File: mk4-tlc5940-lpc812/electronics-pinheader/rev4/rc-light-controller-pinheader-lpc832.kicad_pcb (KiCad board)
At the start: 2 copper layers, 44 x 23 mm, 14 parts, among them J1 Pinheader right-angle 2x17, J2 Pinheader straight 1x06, J3 Pinheader straight 1x06, T9 PMV30UN, U1 LPC832M101FDH20, U2 TLC5940PWP, U3 MCP1703A-3302_SOT23

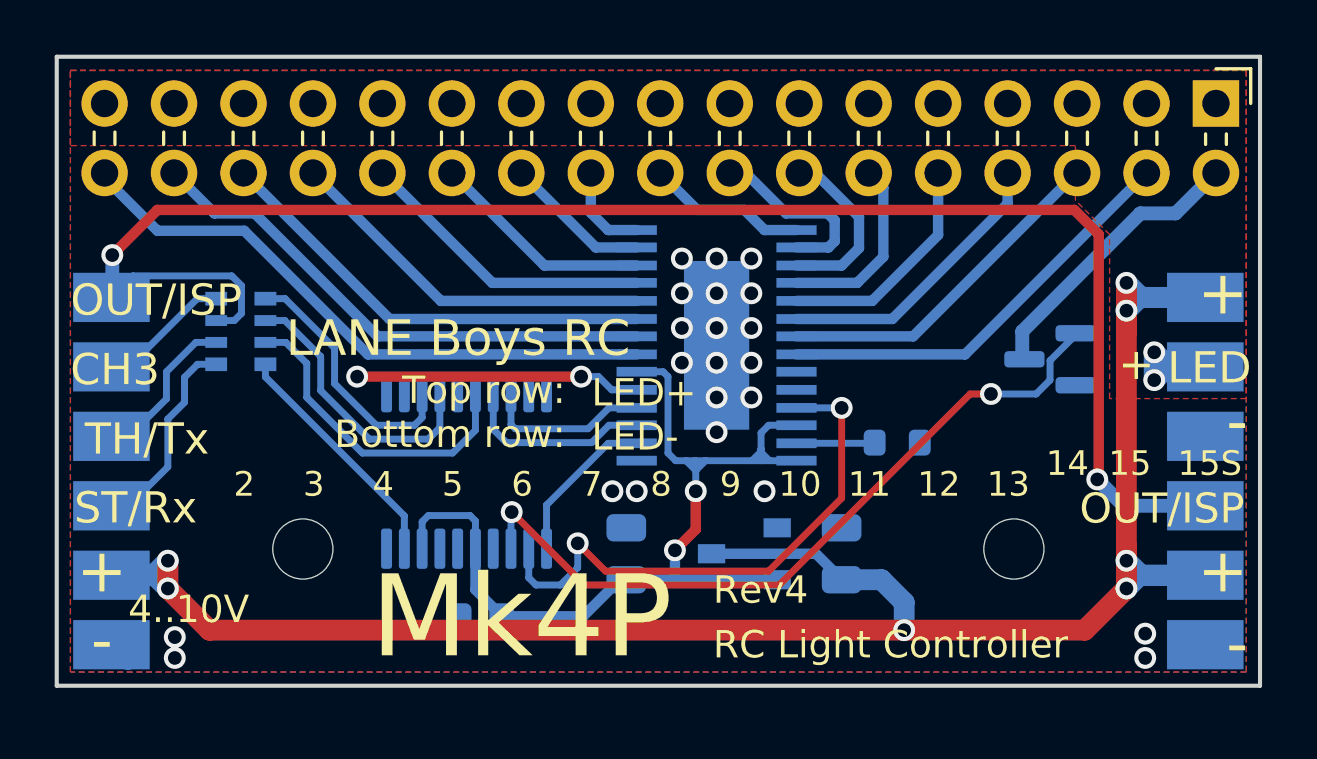
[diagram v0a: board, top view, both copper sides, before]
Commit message: Fix layout and pass DRC
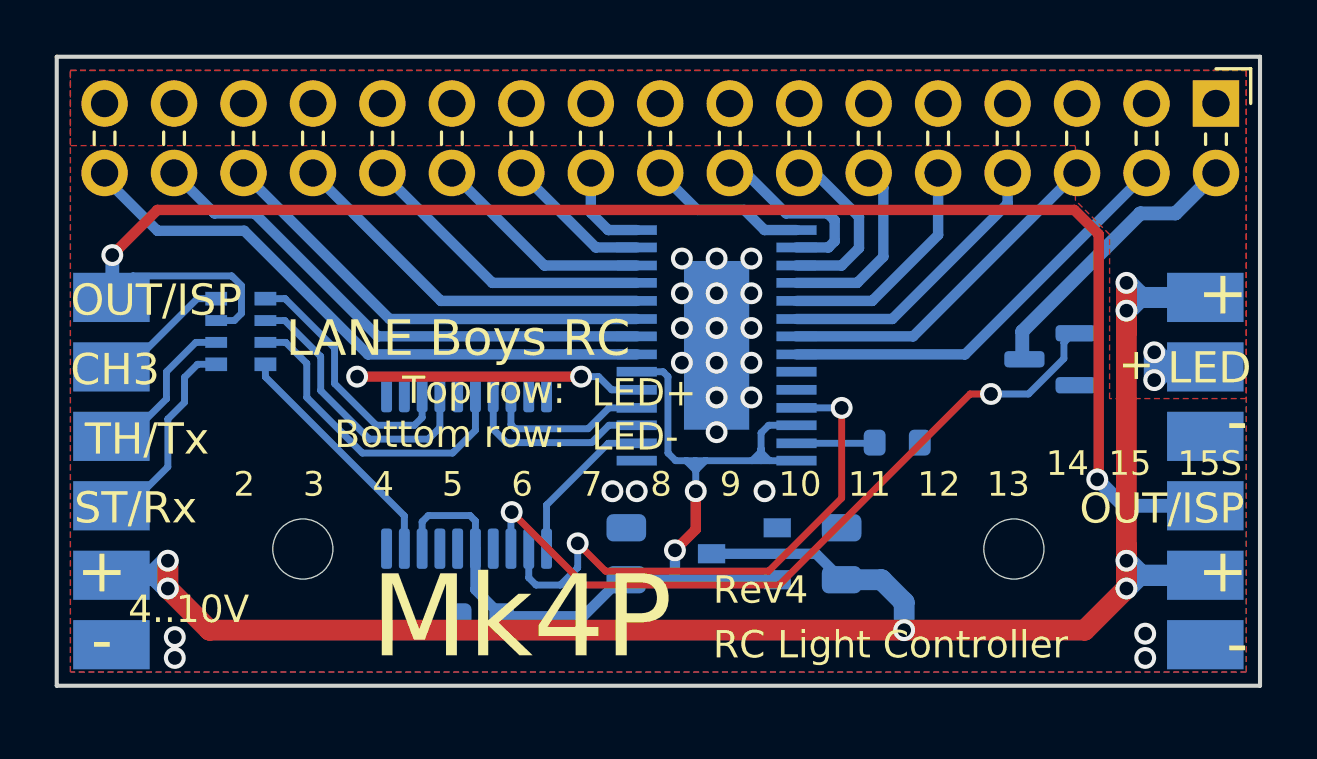
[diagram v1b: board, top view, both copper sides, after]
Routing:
- net /OUT-ISP-out: track 61.9 -> 59.3 mm
- net GND: track 1.85 -> 0.21 mm
- net /CH3-in: track 4.94 -> 4.22 mm
- net /ST-Rx-in: track 7.57 -> 6.89 mm
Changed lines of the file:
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@@
     (fp_line (start 1.042929 28.32) (end 1.497071 28.32) (layer "F.SilkS") (width 0.12))
     (fp_line (start 1.042929 8) (end 1.497071 8) (layer "F.SilkS") (width 0.12))
-    (fp_line (start -1.8 -1.8) (end -1.8 42.45) (layer "F.CrtYd") (width 0.05))
     (fp_line (start -0.32 40.32) (end -0.32 40.96) (layer "F.Fab") (width 0.1))
     (fp_line (start -0.32 2.22) (end -0.32 2.86) (layer "F.Fab") (width 0.1))
@@
   (via (at 157.606 109.047) (size 0.8) (drill 0.5) (layers "F.Cu" "B.Cu") (net 1))
   (segment (start 157.6314 105.7704) (end 157.352 105.491) (width 0.254) (layer "B.Cu") (net 1))
+  (segment (start 150.113 107.777) (end 150.311 107.975) (width 0.254) (layer "B.Cu") (net 1))
+  (segment (start 148.361 108.9885) (end 148.361 108.005) (width 0.254) (layer "B.Cu") (net 1))
   (segment (start 158.368 106.126) (end 158.0124 105.7704) (width 0.254) (layer "B.Cu") (net 1))
   (segment (start 160.4254 105.7704) (end 158.7236 105.7704) (width 0.254) (layer "B.Cu") (net 1))
   (segment (start 161.3398 110.1138) (end 155.8303 110.1138) (width 0.381) (layer "B.Cu") (net 1))
+  (segment (start 148.589 107.777) (end 150.113 107.777) (width 0.254) (layer "B.Cu") (net 1))
   (segment (start 161.035 104.475) (end 160.7556 104.7544) (width 0.254) (layer "B.Cu") (net 1))
   (segment (start 154.2532 111.46) (end 155.6017 110.1115) (width 0.381) (layer "B.Cu") (net 1))
   (segment (start 160.7556 105.4402) (end 160.4254 105.7704) (width 0.254) (layer "B.Cu") (net 1))
   (segment (start 160.7556 105.3386) (end 160.7556 105.4402) (width 0.254) (layer "B.Cu") (net 1))
-  (segment (start 150.113 107.777) (end 150.311 107.975) (width 0.254) (layer "B.Cu") (net 1))
-  (segment (start 148.361 108.9885) (end 148.361 108.692) (width 0.254) (layer "B.Cu") (net 1))
   (segment (start 160.7556 105.4656) (end 161.0604 105.7704) (width 0.254) (layer "B.Cu") (net 1))
   (segment (start 158.368 106.126) (end 158.368 105.7958) (width 0.254) (layer "B.Cu") (net 1))
   (segment (start 158.7236 105.7704) (end 158.3426 105.7704) (width 0.254) (layer "B.Cu") (net 1))
-  (segment (start 148.589 107.777) (end 150.113 107.777) (width 0.254) (layer "B.Cu") (net 1))
   (segment (start 157.352 105.491) (end 157.352 102.697) (width 0.254) (layer "B.Cu") (net 1))
-  (segment (start 158.368 106.888) (end 158.368 106.761) (width 0.254) (layer "B.Cu") (net 1))
+  (segment (start 148.361 108.005) (end 148.589 107.777) (width 0.254) (layer "B.Cu") (net 1))
   (segment (start 157.352 102.697) (end 157.1742 102.5192) (width 0.254) (layer "B.Cu") (net 1))
+  (segment (start 158.368 106.888) (end 158.368 106.126) (width 0.254) (layer "B.Cu") (net 1))
   (segment (start 158.0124 105.7704) (end 157.6314 105.7704) (width 0.254) (layer "B.Cu") (net 1))
-  (segment (start 158.368 106.888) (end 158.368 106.126) (width 0.254) (layer "B.Cu") (net 1))
   (segment (start 162.051 105.7704) (end 161.0604 105.7704) (width 0.254) (layer "B.Cu") (net 1))
   (segment (start 155.6017 110.1115) (end 155.828 110.1115) (width 0.381) (layer "B.Cu") (net 1))
@@
   (segment (start 150.311 110.4895) (end 151.2815 111.46) (width 0.381) (layer "B.Cu") (net 1))
   (segment (start 160.7556 105.7704) (end 160.4254 105.7704) (width 0.254) (layer "B.Cu") (net 1))
+  (segment (start 150.311 107.975) (end 150.311 108.9885) (width 0.254) (layer "B.Cu") (net 1))
   (segment (start 157.1742 102.5192) (end 156.209 102.5192) (width 0.254) (layer "B.Cu") (net 1))
-  (segment (start 148.361 108.005) (end 148.589 107.777) (width 0.254) (layer "B.Cu") (net 1))
   (segment (start 151.2815 111.46) (end 154.2532 111.46) (width 0.381) (layer "B.Cu") (net 1))
   (segment (start 158.3426 105.7704) (end 158.0124 105.7704) (width 0.254) (layer "B.Cu") (net 1))
   (segment (start 158.368 106.126) (end 158.7236 105.7704) (width 0.254) (layer "B.Cu") (net 1))
-  (segment (start 148.361 108.9885) (end 148.361 108.005) (width 0.254) (layer "B.Cu") (net 1))
   (segment (start 160.7556 105.3386) (end 160.7556 105.7704) (width 0.254) (layer "B.Cu") (net 1))
-  (segment (start 150.311 107.975) (end 150.311 108.9885) (width 0.254) (layer "B.Cu") (net 1))
   (segment (start 160.7556 104.7544) (end 160.7556 105.3386) (width 0.254) (layer "B.Cu") (net 1))
   (segment (start 158.368 105.7958) (end 158.3426 105.7704) (width 0.254) (layer "B.Cu") (net 1))
@@
   (via (at 160.4 103.459) (size 0.8) (drill 0.5) (layers "F.Cu" "B.Cu") (net 2))
   (segment (start 137.151 112.349) (end 137 112.5) (width 0.762) (layer "B.Cu") (net 2))
-  (segment (start 137.611 113.111) (end 137 112.5) (width 0.635) (layer "B.Cu") (net 2))
-  (segment (start 137.77 112.5) (end 137 112.5) (width 0.635) (layer "B.Cu") (net 2))
   (segment (start 174.116 110.444) (end 174.116 108.92) (width 0.762) (layer "F.Cu") (net 3))
   (segment (start 140.588 111.968) (end 139.064 110.444) (width 0.762) (layer "F.Cu") (net 3))
@@
   (segment (start 139.064 105.999) (end 139.064 104.2464) (width 0.254) (layer "B.Cu") (net 18))
   (segment (start 140.15 102.246) (end 140.831 102.246) (width 0.254) (layer "B.Cu") (net 18))
-  (segment (start 137 107.42) (end 137.643 107.42) (width 0.254) (layer "B.Cu") (net 18))
-  (segment (start 137.024 107.396) (end 137 107.42) (width 0.762) (layer "B.Cu") (net 18))
   (segment (start 139.6736 103.6368) (end 139.6736 102.7224) (width 0.254) (layer "B.Cu") (net 18))
   (segment (start 137.643 107.42) (end 139.064 105.999) (width 0.254) (layer "B.Cu") (net 18))
@@
   (segment (start 140.0864 101.446) (end 140.831 101.446) (width 0.254) (layer "B.Cu") (net 19))
   (segment (start 137 104.88) (end 137.643 104.88) (width 0.254) (layer "B.Cu") (net 19))
-  (segment (start 137 102.34) (end 137.643 102.34) (width 0.254) (layer "B.Cu") (net 20))
-  (segment (start 137 102.34) (end 136.929 102.34) (width 0.381) (layer "B.Cu") (net 20))
   (segment (start 140.137 99.846) (end 140.831 99.846) (width 0.254) (layer "B.Cu") (net 20))
   (segment (start 137.643 102.34) (end 140.137 99.846) (width 0.254) (layer "B.Cu") (net 20))
@@
   (via (at 137.032 98.252) (size 0.8) (drill 0.5) (layers "F.Cu" "B.Cu") (net 21))
   (via (at 173.0492 106.4562) (size 0.8) (drill 0.5) (layers "F.Cu" "B.Cu") (net 21))
-  (segment (start 137.564 99.8) (end 137 99.8) (width 0.254) (layer "B.Cu") (net 21))
   (segment (start 141.7564 99.3696) (end 141.4008 99.014) (width 0.254) (layer "B.Cu") (net 21))
-  (segment (start 137.278 99.522) (end 137 99.8) (width 0.254) (layer "B.Cu") (net 21))
   (segment (start 137.032 98.252) (end 137.032 99.768) (width 0.508) (layer "B.Cu") (net 21))
   (segment (start 137.032 99.768) (end 137 99.8) (width 0.381) (layer "B.Cu") (net 21))
   (segment (start 141.4008 99.014) (end 137.786 99.014) (width 0.254) (layer "B.Cu") (net 21))
-  (segment (start 177 107.42) (end 176.3636 108.0564) (width 0.508) (layer "B.Cu") (net 21))
   (segment (start 141.496 100.646) (end 141.7564 100.3856) (width 0.254) (layer "B.Cu") (net 21))
   (segment (start 173.0492 106.4562) (end 174.013 107.42) (width 0.508) (layer "B.Cu") (net 21))
   (segment (start 174.013 107.42) (end 177 107.42) (width 0.508) (layer "B.Cu") (net 21))
-  (segment (start 137.77 99.8) (end 137 99.8) (width 0.508) (layer "B.Cu") (net 21))
   (segment (start 140.831 100.646) (end 141.496 100.646) (width 0.254) (layer "B.Cu") (net 21))
   (segment (start 137.786 99.014) (end 137 99.8) (width 0.254) (layer "B.Cu") (net 21))
@@
   (via (at 151.637 107.65) (size 0.8) (drill 0.5) (layers "F.Cu" "B.Cu") (net 34))
   (via (at 169.163 103.332) (size 0.8) (drill 0.5) (layers "F.Cu" "B.Cu") (net 34))
-  (segment (start 170.814 103.332) (end 171.322 102.824) (width 0.254) (layer "B.Cu") (net 34))
+  (segment (start 169.163 103.332) (end 170.5346 103.332) (width 0.254) (layer "B.Cu") (net 34))
   (segment (start 151.637 107.65) (end 151.611 107.676) (width 0.254) (layer "B.Cu") (net 34))
-  (segment (start 171.322 102.112) (end 172.322 101.112) (width 0.254) (layer "B.Cu") (net 34))
+  (segment (start 170.5346 103.332) (end 171.83 102.0366) (width 0.254) (layer "B.Cu") (net 34))
   (segment (start 151.611 107.676) (end 151.611 108.9885) (width 0.254) (layer "B.Cu") (net 34))
-  (segment (start 171.322 102.824) (end 171.322 102.112) (width 0.254) (layer "B.Cu") (net 34))
-  (segment (start 169.163 103.332) (end 170.814 103.332) (width 0.254) (layer "B.Cu") (net 34))
+  (segment (start 171.83 101.4524) (end 172.1079 101.1745) (width 0.254) (layer "B.Cu") (net 34))
+  (segment (start 172.1079 101.1745) (end 172.2595 101.1745) (width 0.254) (layer "B.Cu") (net 34))
+  (segment (start 171.83 102.0366) (end 171.83 101.4524) (width 0.254) (layer "B.Cu") (net 34))
   (segment (start 162.051 105.1354) (end 164.9211 105.1354) (width 0.254) (layer "B.Cu") (net 35))
-  (segment (start 164.9211 105.1354) (end 164.9465 105.11) (width 0.254) (layer "B.Cu") (net 35))
   (segment (start 174.624 96.728) (end 175.912 96.728) (width 0.508) (layer "B.Cu") (net 36))
   (segment (start 170.306 101.046) (end 174.624 96.728) (width 0.508) (layer "B.Cu") (net 36))
